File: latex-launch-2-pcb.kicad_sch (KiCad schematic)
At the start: 14 parts, among them J1 Conn_RockBLOCK, J2 Switch_RockBLOCK, J3 Conn_FeatherWeight, J4 Conn_LightAPRS, J5 Conn_MicroSD, J6 Conn_GY-512_MPU6050

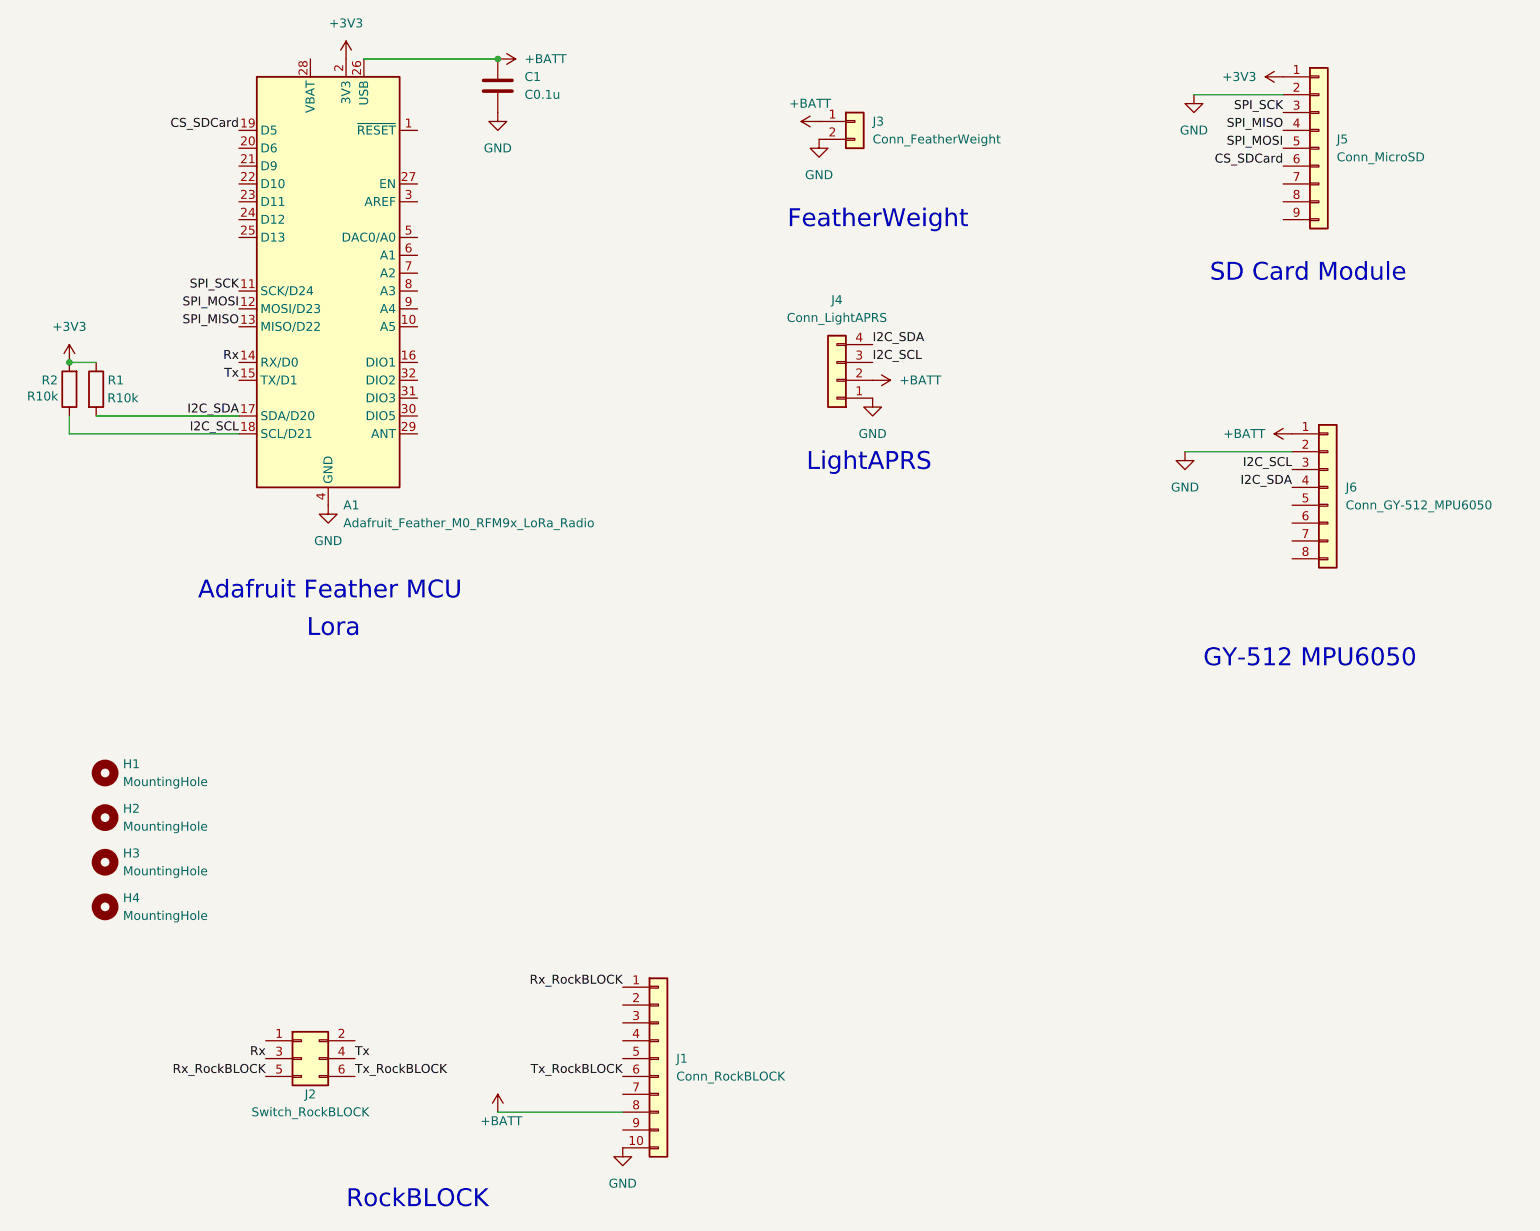
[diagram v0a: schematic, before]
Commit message: PCB version 2
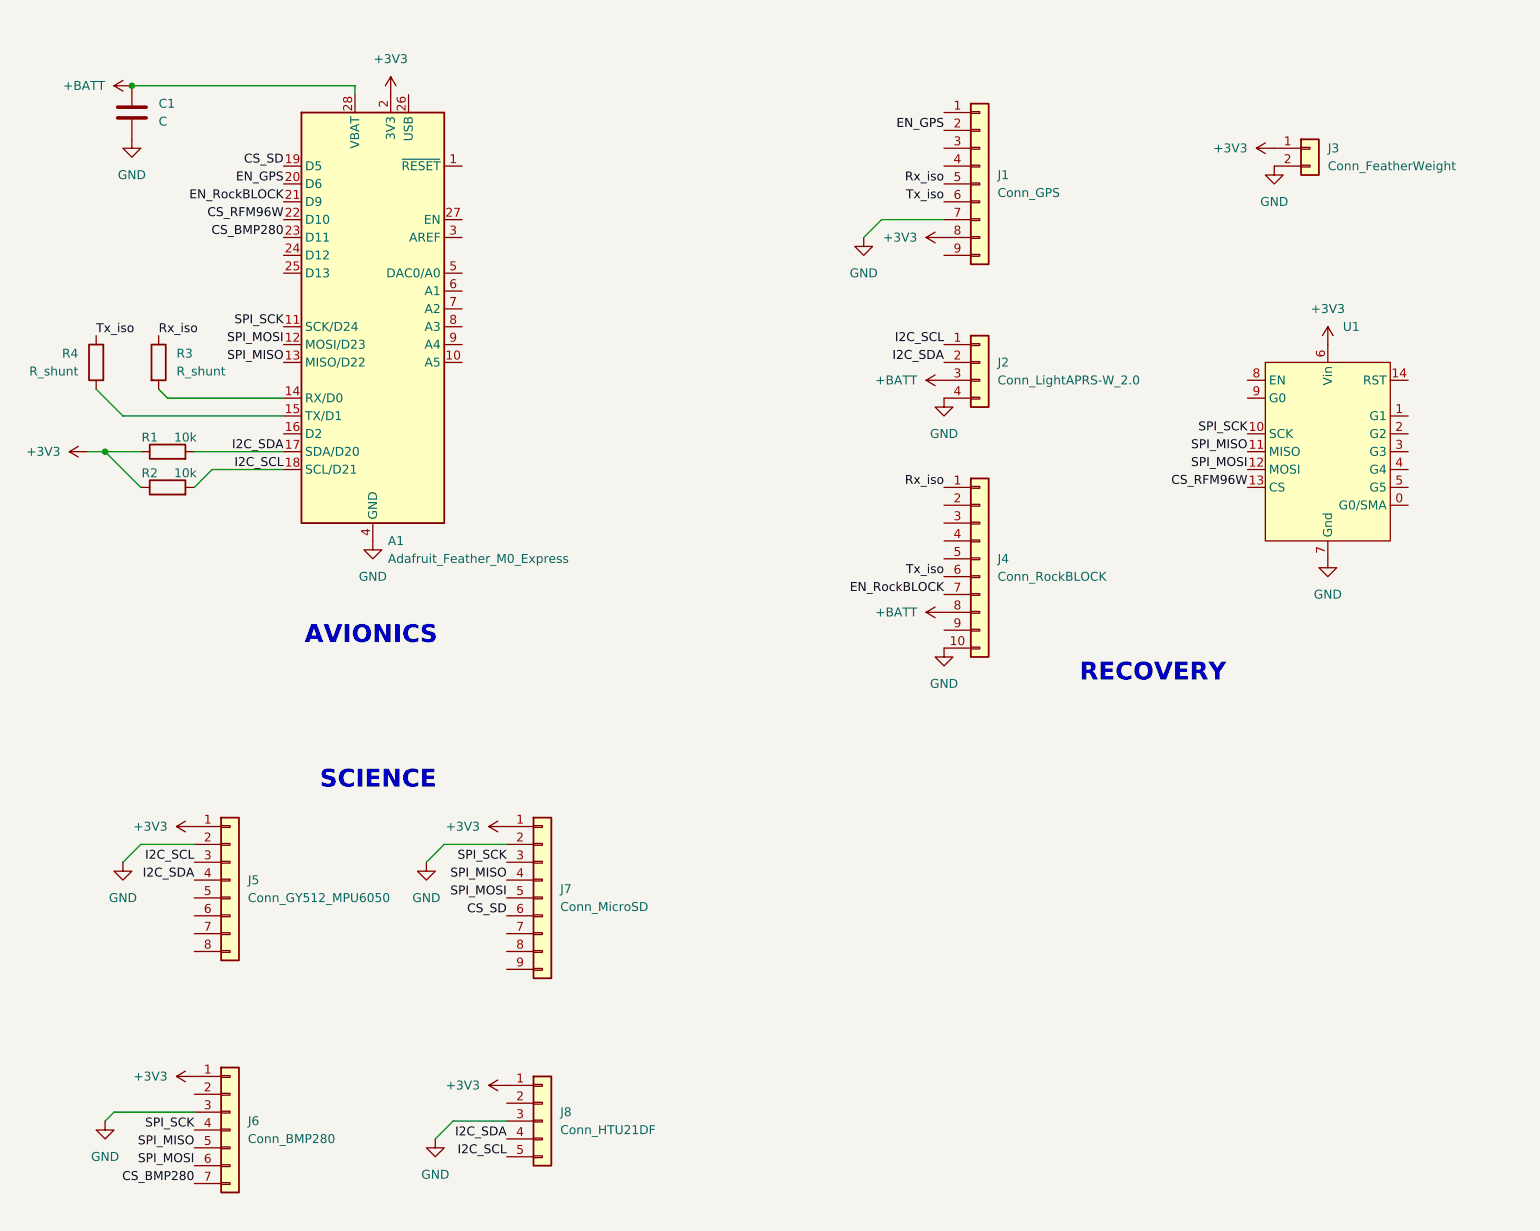
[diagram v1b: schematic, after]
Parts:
- removed A1: Adafruit_Feather_M0_RFM9x_LoRa_Radio, Module:Adafruit_Feather_M0_RFM, symbol MCU_Module:Adafruit_Feather_M0_RFM9x_LoRa_Radio
- removed H1, H2, H3, H4: MountingHole, MountingHole:MountingHole_3.2mm_M3_DIN965_Pad, symbol Mechanical:MountingHole
- removed J1: Conn_RockBLOCK, Connector_Molex:Molex_PicoBlade_53047-1010_1x10_P1.25mm_Vertical, symbol Connector_Generic:Conn_01x10
- removed J2: Switch_RockBLOCK, Connector_PinSocket_2.54mm:PinSocket_2x03_P2.54mm_Vertical, symbol Connector_Generic:Conn_02x03_Odd_Even
- removed J4: Conn_LightAPRS, Connector_JST:JST_PH_S4B-PH-SM4-TB_1x04-1MP_P2.00mm_Horizontal, symbol Connector_Generic:Conn_01x04
- removed J5: Conn_MicroSD, Module:Adafruit_MicroSD_Breakout, symbol Connector_Generic:Conn_01x09
- removed J6: Conn_GY-512_MPU6050, Module:GY-521 MPU6050, symbol Connector_Generic:Conn_01x08
- added A1: Adafruit_Feather_M0_Express, Module:Adafruit_Feather_M0_RFM_WithMountingHoles, symbol MCU_Module:Adafruit_Feather_M0_Express
- added J1: Conn_GPS, Latex Launch 2 Footprints:Adafruit_GPS_Breakout, symbol Connector_Generic:Conn_01x09
- added J2: Conn_LightAPRS-W_2.0, Connector_JST:JST_PH_S4B-PH-SM4-TB_1x04-1MP_P2.00mm_Horizontal, symbol Connector_Generic:Conn_01x04
- added J4: Conn_RockBLOCK, Connector_Molex:Molex_PicoBlade_53047-1010_1x10_P1.25mm_Vertical, symbol Connector_Generic:Conn_01x10
- added J5: Conn_GY512_MPU6050, Latex Launch 2 Footprints:GY-521 MPU6050, symbol Connector_Generic:Conn_01x08
- added J6: Conn_BMP280, Latex Launch 2 Footprints:Adafruit_BMP280_Breakout, symbol Connector_Generic:Conn_01x07
- added J7: Conn_MicroSD, Latex Launch 2 Footprints:Adafruit_MicroSD_Breakout, symbol Connector_Generic:Conn_01x09
- added J8: Conn_HTU21DF, Latex Launch 2 Footprints:Adafruit_HTU21DF_Breakout, symbol Connector_Generic:Conn_01x05
- added R3, R4: R_shunt, Connector_PinHeader_2.54mm:PinHeader_1x02_P2.54mm_Vertical, symbol Device:R
- added U1: ~, Latex Launch 2 Footprints:Adafruit_RFM96W_LoRa_Breakout, symbol adafruit_rfm96w_lora_breakout:Adafruit_RFM96W_LoRa_Breakout
- C1: value C0.1u -> C; footprint Capacitor_THT:C_Rect_L7.0mm_W2.5mm_P5.00mm -> Capacitor_THT:C_Rect_L4.6mm_W2.0mm_P2.50mm_MKS02_FKP02
- R1, R2: value R10k -> 10k
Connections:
- net +3V3: now also J3.1 (Pin_1), R2.1, A1.2 (3V3), J1.8 (Pin_8), J5.1 (Pin_1), J6.1 (Pin_1), J7.1 (Pin_1), J8.1 (Pin_1), U1.6 (Vin); no longer R2.2
- net +BATT: now also A1.28 (VBAT), J2.3 (Pin_3), J4.8 (Pin_8); no longer J3.1 (Pin_1)
- net GND: now also A1.4 (GND), J1.7 (Pin_7), J2.4 (Pin_4), J4.10 (Pin_10), J5.2 (Pin_2), J6.3 (Pin_3), J7.2 (Pin_2), J8.3 (Pin_3), U1.7 (Gnd)
- net I2C_SCL: now also R2.2, A1.18 (SCL/D21), J2.1 (Pin_1), J5.3 (Pin_3), J8.5 (Pin_5); no longer R2.1
- net I2C_SDA: now also A1.17 (SDA/D20), J2.2 (Pin_2), J5.4 (Pin_4), J8.4 (Pin_4)
- net SPI_MISO: now also A1.13 (MISO/D22), J6.5 (Pin_5), J7.4 (Pin_4), U1.11 (MISO)
- net SPI_MOSI: now also A1.12 (MOSI/D23), J6.6 (Pin_6), J7.5 (Pin_5), U1.12 (MOSI)
- net SPI_SCK: now also A1.11 (SCK/D24), J6.4 (Pin_4), J7.3 (Pin_3), U1.10 (SCK)
- new net: A1.14 (RX/D0), R3.2
- new net: A1.15 (TX/D1), R4.2
- new net CS_BMP280: A1.23 (D11), J6.7 (Pin_7)
- new net CS_RFM96W: A1.22 (D10), U1.13 (CS)
- new net CS_SD: A1.19 (D5), J7.6 (Pin_6)
- new net EN_GPS: A1.20 (D6), J1.2 (Pin_2)
- new net EN_RockBLOCK: A1.21 (D9), J4.7 (Pin_7)
- new net Rx_iso: J1.5 (Pin_5), J4.1 (Pin_1), R3.1
- new net Tx_iso: J1.6 (Pin_6), J4.6 (Pin_6), R4.1
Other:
- note added: "AVIONICS"
- note added: "RECOVERY"
- note added: "SCIENCE"
- note removed: "Adafruit Feather MCU"
- note removed: "FeatherWeight"
- note removed: "GY-512 MPU6050"
- note removed: "LightAPRS"
- note removed: "Lora"
- note removed: "RockBLOCK"
- note removed: "SD Card Module"
- company: (none) -> Stanford Student Space Initiative
- title: (none) -> Balloons 2025-26 Latex Launch 2
